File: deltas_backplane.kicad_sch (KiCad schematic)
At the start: 11 parts, among them J1 SNP_female_straight, J2 SNP_female_straight, J3 SNP_female_straight, J4 SNP_female_straight, J5 SNP_male_angle, J6 zx_bus, J7 zx_bus, J8 Barrel_Jack, SW1 SW_SPDT

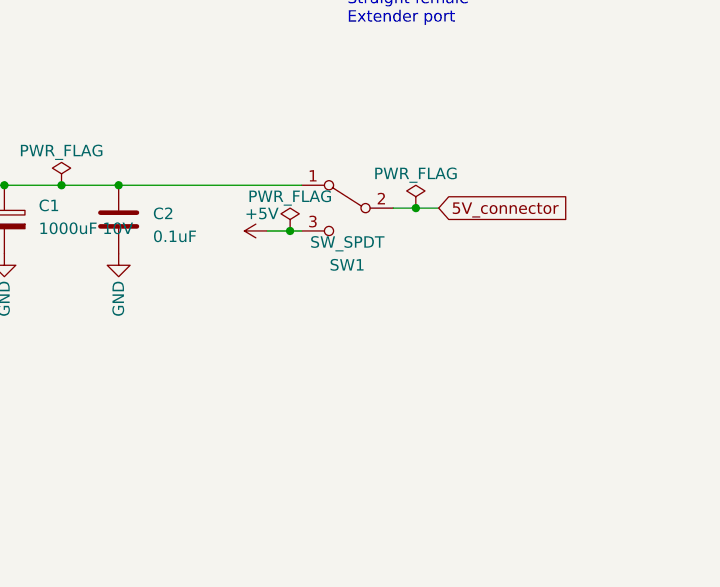
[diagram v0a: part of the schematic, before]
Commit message: 03.10.2023 update
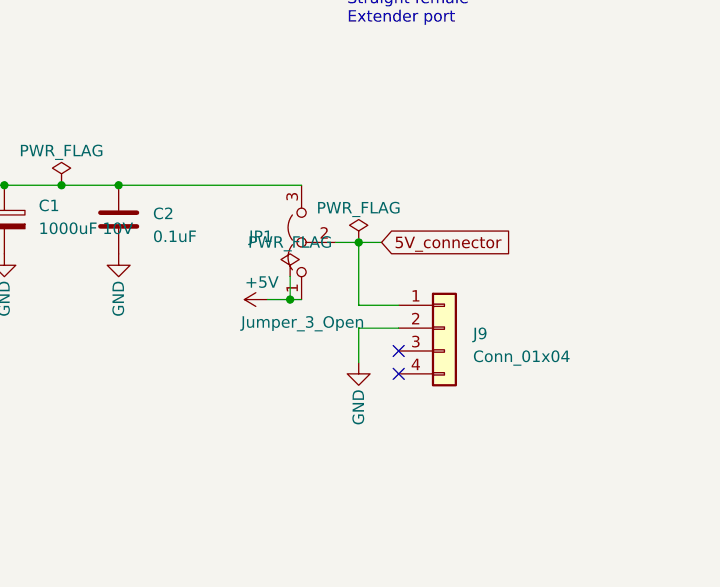
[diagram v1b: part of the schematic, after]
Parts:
- removed SW1: SW_SPDT, Backplane:MTS-102-C3, symbol Switch:SW_SPDT
- added J9: Conn_01x04, Connector_PinHeader_2.54mm:PinHeader_1x04_P2.54mm_Vertical, symbol Connector_Generic:Conn_01x04
- added JP1: Jumper_3_Open, Connector_PinHeader_2.54mm:PinHeader_1x03_P2.54mm_Vertical, symbol Jumper:Jumper_3_Open
- C1: footprint Capacitor_THT:CP_Radial_Tantal_D7.0mm_P5.00mm -> Capacitor_THT:CP_Radial_D8.0mm_P5.00mm; symbol Device:C_Polarized -> backplane_2:C_Polarized
- C2: symbol Device:C -> backplane_2:C
- J1, J2, J3, J4: symbol backplane:SNP_female_straight -> backplane_2:SNP_female_straight
- J5: symbol backplane:SNP_male_angle -> backplane_2:SNP_male_angle
- J6, J7: symbol backplane:zx_bus -> backplane_2:zx_bus
- J8: symbol Connector:Barrel_Jack -> backplane_2:Barrel_Jack
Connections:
- net +5V: now also JP1.1 (A)
- net 5V_connector: now also J9.1 (Pin_1), JP1.2 (C)
- net GND: now also J9.2 (Pin_2)
- net at C1.1, C2.1, J8.1: now also JP1.3 (B)
- no-connect marks 12 -> 14
